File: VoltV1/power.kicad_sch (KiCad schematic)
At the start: 3 parts, among them J1 USBC

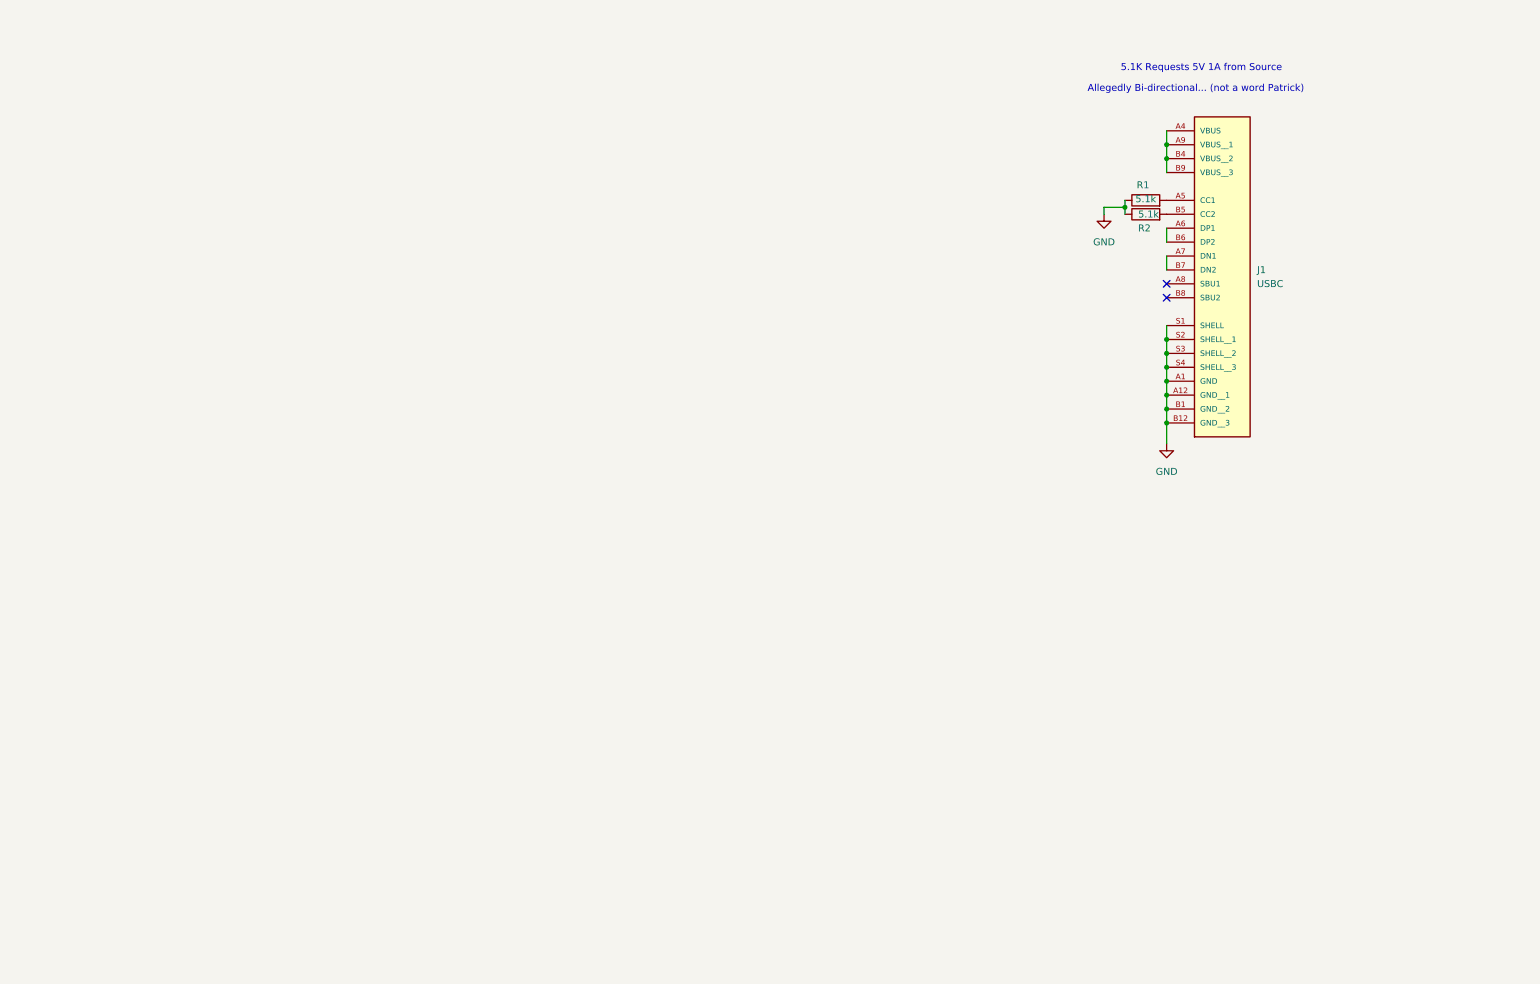
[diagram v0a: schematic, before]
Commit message: merging. power stuff incomplete
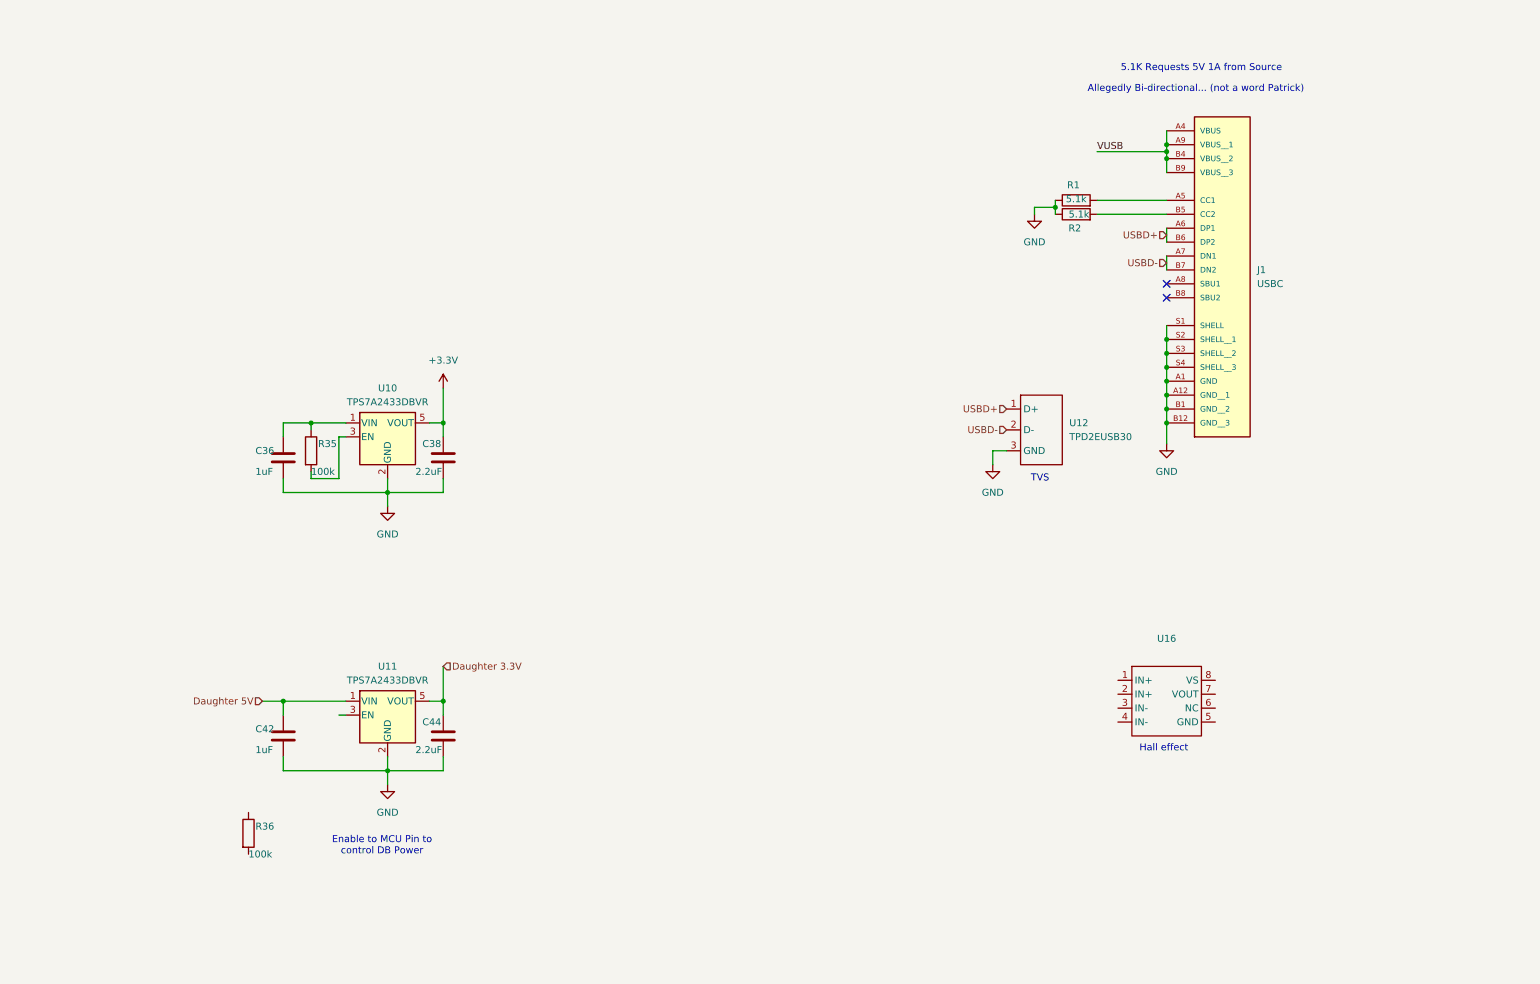
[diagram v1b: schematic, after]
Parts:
- added C36, C42: 1uF, Capacitor_SMD:C_0603_1608Metric, symbol Device:C
- added C38, C44: 2.2uF, Capacitor_SMD:C_0603_1608Metric, symbol Device:C
- added R35, R36: 100k, Resistor_SMD:R_0603_1608Metric, symbol Device:R
- added U10, U11: TPS7A2433DBVR, Package_TO_SOT_SMD:SOT-23-5, symbol Regulator_Linear:AP2112K-3.3
- added U12: TPD2EUSB30, Package_TO_SOT_SMD:Texas_DRT-3, symbol VOLTV1:TPD2EUSB30
- added U16: ~, Package_SO:SOIC-8_3.9x4.9mm_P1.27mm, symbol VOLTV1:TMCS1108A1B
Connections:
- net GND: now also C36.2, C38.2, C42.2, C44.2, U10.2 (GND), U11.2 (GND), U12.3 (GND)
- net VUSB: now reaches J1.A4 (VBUS), J1.A9 (VBUS__1), J1.B4 (VBUS__2), J1.B9 (VBUS__3)
- net USBD+: now reaches J1.A6 (DP1), J1.B6 (DP2)
- net USBD+: now also U12.1 (D+)
- net USBD-: now reaches J1.A7 (DN1), J1.B7 (DN2)
- net USBD-: now also U12.2 (D-)
- new net: C36.1, R35.1, U10.1 (VIN)
- new net: R35.2, U10.3 (EN)
- new net +3.3V: C38.1, U10.5 (VOUT)
- new net Daughter 3.3V: C44.1, U11.5 (VOUT)
- new net Daughter 5V: C42.1, U11.1 (VIN)
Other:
- note added: "Enable to MCU Pin to control DB Power"
- note added: "Hall effect"
- note added: "TVS"
- moved on the sheet: R1, R2

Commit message: updates to schematic
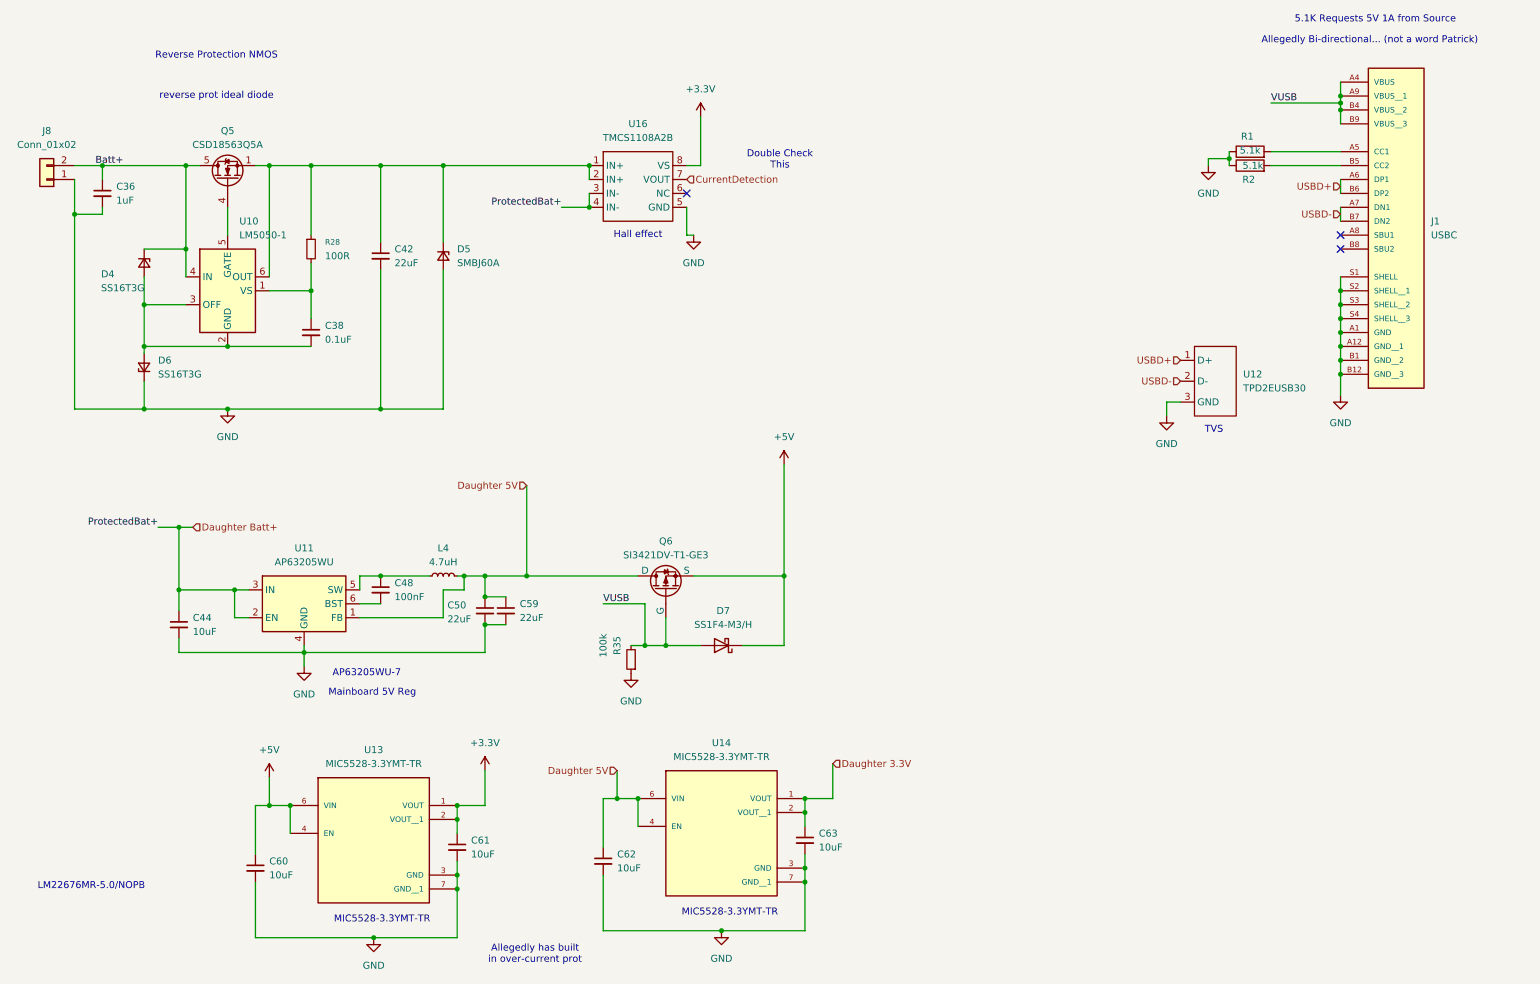
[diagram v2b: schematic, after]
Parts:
- removed C36, C42: 1uF, Capacitor_SMD:C_0603_1608Metric, symbol Device:C
- removed C38, C44: 2.2uF, Capacitor_SMD:C_0603_1608Metric, symbol Device:C
- removed R35, R36: 100k, Resistor_SMD:R_0603_1608Metric, symbol Device:R
- removed U10, U11: TPS7A2433DBVR, Package_TO_SOT_SMD:SOT-23-5, symbol Regulator_Linear:AP2112K-3.3
- added C36: 1uF, symbol Device:C_Small
- added C38: 0.1uF, symbol Device:C_Small
- added C42, C50, C59: 22uF, symbol Device:C_Small
- added C44, C60, C61, C62, C63: 10uF, symbol Device:C_Small
- added C48: 100nF, symbol Device:C_Small
- added D4, D6: SS16T3G, symbol Device:D_Zener_Small
- added D5: SMBJ60A, symbol Device:D_Zener_Small
- added D7: SS1F4-M3/H, Diode_SMD:D_SOD-123, symbol Device:D_Schottky
- added J8: Conn_01x02, symbol Connector_Generic:Conn_01x02
- added L4: 4.7uH, symbol Device:L_Small
- added Q5: CSD18563Q5A, Package_TO_SOT_SMD:TDSON-8-1, symbol Transistor_FET:CSD18563Q5A
- added Q6: SI3421DV-T1-GE3, Package_SO:TSOP-6_1.65x3.05mm_P0.95mm, symbol Simulation_SPICE:PMOS
- added R28: 100R, symbol Device:R_Small
- added R35: 100k, Resistor_SMD:R_0603_1608Metric, symbol Device:R_Small
- added U10: LM5050-1, Package_TO_SOT_SMD:TSOT-23-6, symbol Power_Management:LM5050-1
- added U11: AP63205WU, Package_TO_SOT_SMD:TSOT-23-6, symbol Regulator_Switching:AP63205WU
- added U13, U14: MIC5528-3.3YMT-TR, VOLTV1:SON40P120X120X60-7N, symbol VOLTV1:MIC5528-3.3YMT-TR
- U16: value ~ -> TMCS1108A2B
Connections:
- net +3.3V: now also U16.8 (VS), C61.1, U13.1 (VOUT), U13.2 (VOUT__1)
- net Daughter 3.3V: now also C63.1, U14.1 (VOUT), U14.2 (VOUT__1)
- net Daughter 5V: now also C50.1, C59.1, C62.1, L4.2, Q6.1 (D), Q6.2 (D), Q6.5 (D), Q6.6 (D), U11.1 (FB), U14.4 (EN), U14.6 (VIN)
- net GND: now also U16.5 (GND), C36.2, C42.2, C44.2, C50.2, C59.2, C60.2, C61.2, C62.2, C63.2, D5.2 (A), D6.1 (K), J8.1 (Pin_1), R35.1, U11.4 (GND), U13.3 (GND), U13.7 (GND__1), U14.3 (GND), U14.7 (GND__1)
- net VUSB: now also D7.2 (A), Q6.3 (G), R35.2
- net at U16.1 (IN+): now also U16.2 (IN+), C42.1, D5.1 (K), Q5.1 (S), Q5.2 (S), Q5.3 (S), R28.1, U10.6 (OUT)
- net Daughter Batt+: now reaches U16.3 (IN-)
- net Daughter Batt+: now also U16.4 (IN-), C44.1, U11.2 (EN), U11.3 (IN)
- net CurrentDetection: now reaches U16.7 (VOUT)
- new net: C38.1, R28.2, U10.1 (VS)
- new net: C38.2, D4.2 (A), D6.2 (A), U10.2 (GND), U10.3 (OFF)
- new net: C48.1, L4.1, U11.5 (SW)
- new net: C48.2, U11.6 (BST)
- new net: Q5.4 (G), U10.5 (GATE)
- new net +5V: C60.1, D7.1 (K), Q6.4 (S), U13.4 (EN), U13.6 (VIN)
- new net Batt+: C36.1, D4.1 (K), J8.2 (Pin_2), Q5.5 (D), U10.4 (IN)
- no-connect marks 2 -> 3
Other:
- note added: "AP63205WU-7"
- note added: "Allegedly has built in over-current prot"
- note added: "Double Check This"
- note added: "LM22676MR-5.0/NOPB"
- note added: "MIC5528-3.3YMT-TR"
- note added: "Mainboard 5V Reg"
- note added: "Reverse Protection NMOS"
- note added: "reverse prot ideal diode"
- note removed: "Enable to MCU Pin to control DB Power"
- moved on the sheet: J1, R1, R2, U12, U16

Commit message: schematic updates
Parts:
- C36, C38, C42, C44, C48, C50, C59, C60, C61, C62, C63: footprint (none) -> Capacitor_SMD:C_0402_1005Metric
- L4: footprint (none) -> Inductor_SMD:L_0603_1608Metric
- R1, R2, R35: footprint Resistor_SMD:R_0603_1608Metric -> Resistor_SMD:R_0402_1005Metric
- R28: footprint (none) -> Resistor_SMD:R_0402_1005Metric
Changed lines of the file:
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@@
 			)
 		)
-		(property "Footprint" ""
+		(property "Footprint" "Capacitor_SMD:C_0402_1005Metric"
 			(at 66.04 76.2 0)
 			(effects
@@
 			)
 		)
-		(property "Footprint" ""
+		(property "Footprint" "Capacitor_SMD:C_0402_1005Metric"
 			(at 78.74 123.19 0)
 			(effects
@@
 			)
 		)
-		(property "Footprint" ""
+		(property "Footprint" "Capacitor_SMD:C_0402_1005Metric"
 			(at 92.71 170.18 0)
 			(effects
@@
 			)
 		)
-		(property "Footprint" ""
+		(property "Footprint" "Capacitor_SMD:C_0402_1005Metric"
 			(at 41.91 129.54 0)
 			(effects
@@
 			)
 		)
-		(property "Footprint" "Resistor_SMD:R_0603_1608Metric"
+		(property "Footprint" "Resistor_SMD:R_0402_1005Metric"
 			(at 237.49 44.958 90)
 			(effects
@@
 			)
 		)
-		(property "Footprint" ""
+		(property "Footprint" "Capacitor_SMD:C_0402_1005Metric"
 			(at 78.74 62.23 0)
 			(effects
@@
 			)
 		)
-		(property "Footprint" "Resistor_SMD:R_0603_1608Metric"
+		(property "Footprint" "Resistor_SMD:R_0402_1005Metric"
 			(at 237.49 47.498 90)
 			(effects
@@
 			)
 		)
-		(property "Footprint" ""
+		(property "Footprint" "Capacitor_SMD:C_0402_1005Metric"
 			(at 119.38 172.72 0)
 			(effects
@@
 			)
 		)
-		(property "Footprint" ""
+		(property "Footprint" "Resistor_SMD:R_0402_1005Metric"
 			(at 66.04 60.96 0)
 			(effects
@@
 			)
 		)
-		(property "Footprint" "Resistor_SMD:R_0603_1608Metric"
+		(property "Footprint" "Resistor_SMD:R_0402_1005Metric"
 			(at 124.46 135.89 0)
 			(effects
@@
 			)
 		)
-		(property "Footprint" ""
+		(property "Footprint" "Capacitor_SMD:C_0402_1005Metric"
 			(at 156.21 168.91 0)
 			(effects
@@
 			)
 		)
-		(property "Footprint" ""
+		(property "Footprint" "Capacitor_SMD:C_0402_1005Metric"
 			(at 55.88 173.99 0)
 			(effects
@@
 			)
 		)
-		(property "Footprint" ""
+		(property "Footprint" "Capacitor_SMD:C_0402_1005Metric"
 			(at 27.94 50.8 0)
 			(effects
@@
 			)
 		)
-		(property "Footprint" ""
+		(property "Footprint" "Capacitor_SMD:C_0402_1005Metric"
 			(at 101.6 127 0)
 			(effects
@@
 			)
 		)
-		(property "Footprint" ""
+		(property "Footprint" "Inductor_SMD:L_0603_1608Metric"
 			(at 90.17 120.65 0)
 			(effects
@@
 			)
 		)
-		(property "Footprint" ""
+		(property "Footprint" "Capacitor_SMD:C_0402_1005Metric"
 			(at 97.79 127 0)
 			(effects
